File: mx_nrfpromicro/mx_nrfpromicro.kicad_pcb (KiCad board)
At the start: 2 copper layers, 22 parts, among them SW1 SW_Push_45deg, SW10 SW_Push_45deg, SW11 SW_Push_45deg, SW12 SW_Push_45deg, SW13 SW_Push_45deg, SW14 SW_Push_45deg, SW15 SW_Push_45deg, SW16 SW_Push_45deg, SW17 SW_Push_45deg, SW2 SW_Push_45deg, SW3 SW_Push_45deg, SW4 SW_Push_45deg, SW5 SW_Push_45deg, SW6 SW_Push_45deg, SW7 SW_Push_45deg, SW8 SW_Push_45deg, SW9 SW_Push_45deg, U1 Nice_Nano_V2

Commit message: updated
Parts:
- SW18: value ~ -> SW_SPDT
- SW19: value ~ -> SW_PUSH
- moved SW11 292.3 mm to (38.1, 90.8)
- moved SW13 278.2 mm to (76.2, 75.8)
- moved SW7 275.9 mm to (57.1, 59.8)
- moved SW1 275.3 mm to (38.1, 52.7)
- moved SW6 274.6 mm to (38.1, 71.8)
- moved SW12 273.7 mm to (57.1, 78.8)
- moved SW14 258.2 mm to (95.2, 83.8)
- moved SW8 254.9 mm to (76.2, 56.8)
- moved SW2 254.5 mm to (57.1, 40.7)
- moved SW16 249.9 mm to (102.1, 105.9), turned to -12 degrees
- moved SW18 249.2 mm to (136.5, 88.7), turned to -90 degrees
- moved TP2 245.5 mm to (125.6, 39.7)
- moved SW19 244.8 mm to (140.6, 76.7), turned to 90 degrees
- moved SW15 237.2 mm to (114.3, 86.0)
- moved U1 236.2 mm to (133.1, 56.0)
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
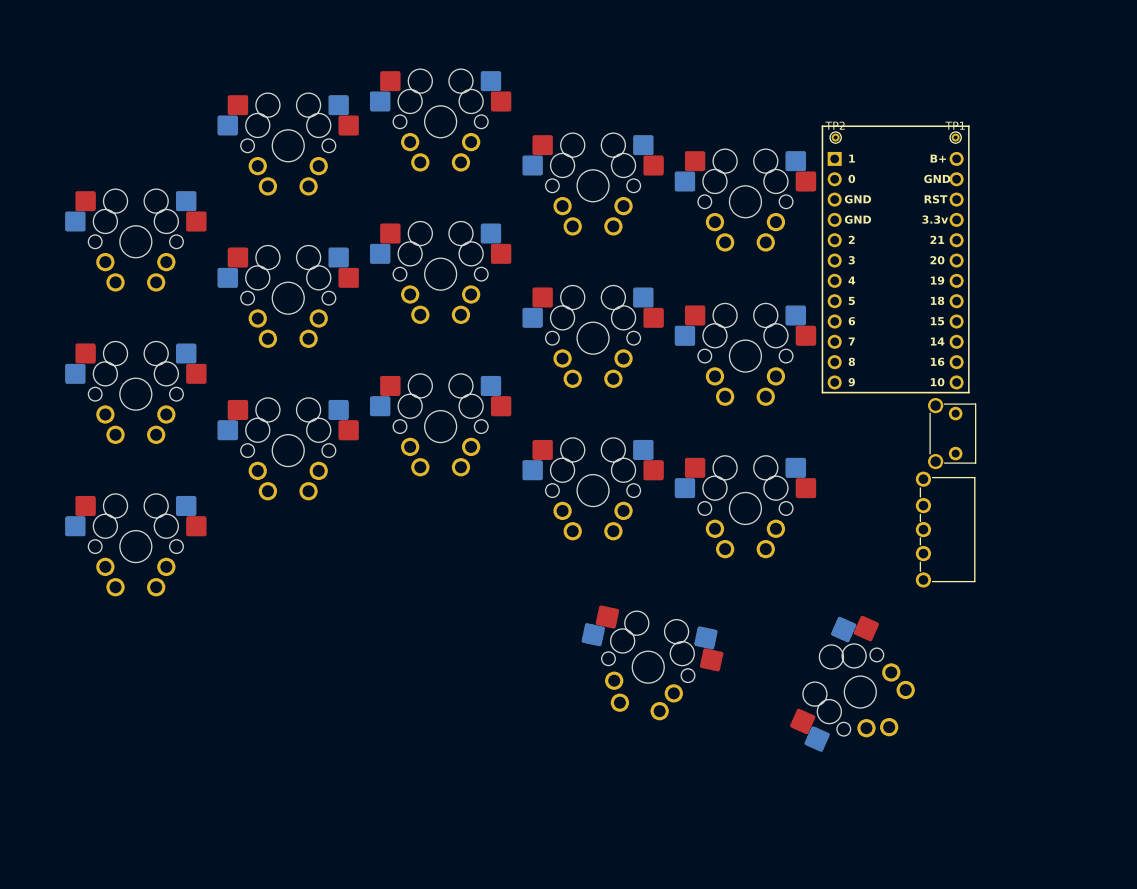
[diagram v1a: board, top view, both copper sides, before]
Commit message: updated
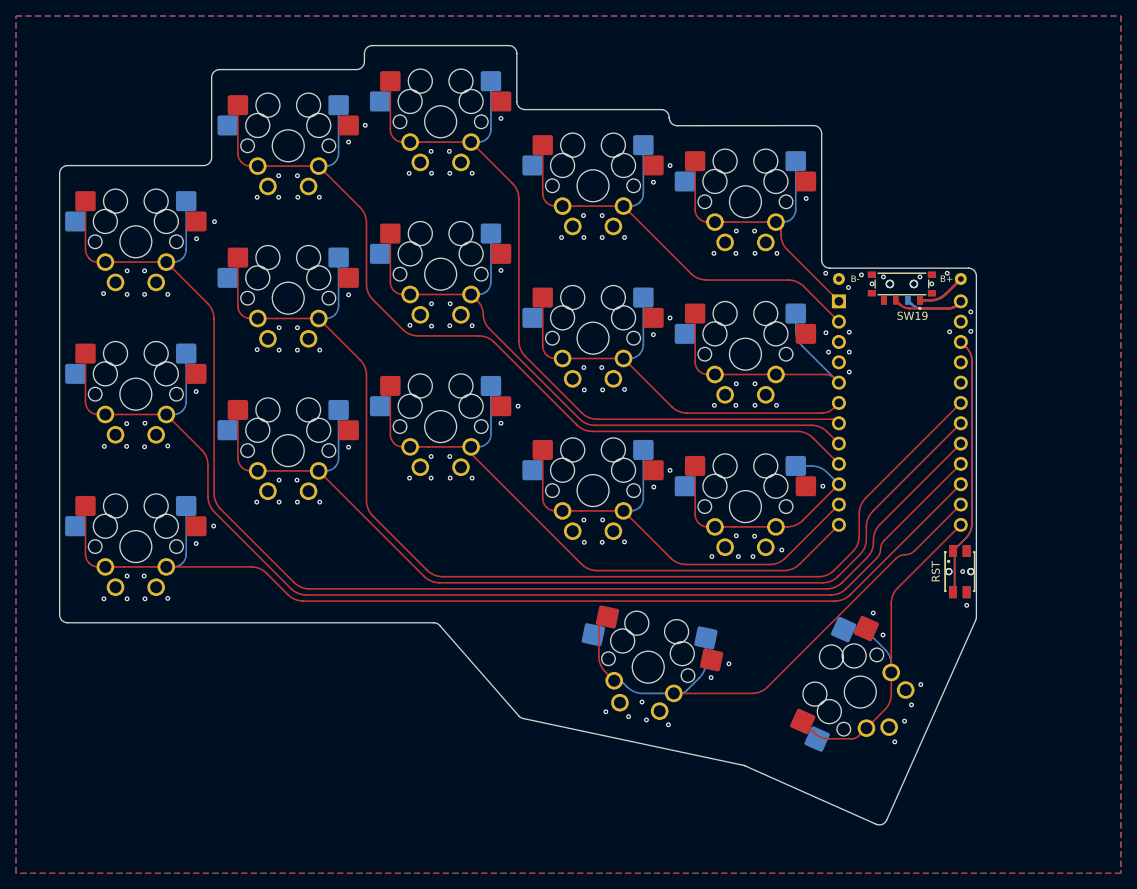
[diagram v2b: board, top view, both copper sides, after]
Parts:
- added RST: 436331045822, BLE_KBD:4363X10458XX, F.Cu at (141.1, 93.9)
- added RST: 436331045822, BLE_KBD:4363X10458XX, B.Cu at (141.1, 93.9)
- B+: renamed from TP1; footprint TestPoint:TestPoint_THTPad_D1.0mm_Drill0.5mm -> TestPoint:TestPoint_THTPad_D1.5mm_Drill0.7mm
- B-: renamed from TP2; footprint TestPoint:TestPoint_THTPad_D1.0mm_Drill0.5mm -> TestPoint:TestPoint_THTPad_D1.5mm_Drill0.7mm
- SW1, SW10, SW11, SW12, SW13, SW14, SW15, SW2, SW3, SW4, SW5, SW6, SW7, SW8, SW9: footprint BLE_KBD:MX_Optional_Reversible_1u -> BLE_KBD:MX_Reversible_Optional_1u
- SW16, SW17: footprint BLE_KBD:MX_Optional_Reversible_1.5u -> BLE_KBD:MX_Reversible_Optional_1.5u
- SW18: value SW_SPDT -> MLL1200S; footprint BLE_KBD:SS12F23G5 -> BLE_KBD:SW_MLL1200S; moved to B.Cu
- SW19: value SW_PUSH -> MLL1200S; footprint BLE_KBD:SW_SIDE_MOUNT -> BLE_KBD:SW_MLL1200S
- moved SW18 30.8 mm to (133.9, 58.0), turned to 0 degrees
- moved SW19 19.9 mm to (133.9, 58.0), turned to 180 degrees
- moved U1 17.8 mm to (133.6, 73.8)
- moved B+ 17.7 mm to (141.2, 57.4)
- moved B- 17.7 mm to (126.0, 57.4)
- moved SW10 0.24 mm to (114.3, 66.8)
- moved SW15 0.24 mm to (114.3, 85.8)
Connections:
- B+ pad 1: Net-(SW18-Pad2) -> Net-(SW18-Pad3)
- SW18 pad 1: Net-(U1-B+) -> unconnected-(SW18-Pad1)
- SW18 pad 2: Net-(SW18-Pad2) -> B+
- SW18 pad 3: unconnected-(SW18-Pad3) -> Net-(SW18-Pad3)
- SW19 pad 1: RST -> Net-(SW18-Pad3)
- SW19 pad 2: GND -> B+
- SW19 pad 3: GND -> unconnected-(SW19-Pad3)
- U1 pad 1: SW1 -> SW5
- U1 pad 10: SW8 -> SW15
- U1 pad 11: SW9 -> SW14
- U1 pad 12: SW10 -> SW13
- U1 pad 13: SW11 -> SW17
- U1 pad 14: SW12 -> SW16
- U1 pad 15: SW13 -> SW11
- U1 pad 16: SW14 -> SW6
- U1 pad 17: SW15 -> SW1
- U1 pad 18: SW16 -> SW12
- U1 pad 19: SW17 -> SW7
- U1 pad 2: SW2 -> SW4
- U1 pad 24: Net-(U1-B+) -> B+
- U1 pad 5: SW3 -> SW10
- U1 pad 6: SW4 -> SW9
- U1 pad 7: SW5 -> SW3
- U1 pad 8: SW6 -> SW8
- U1 pad 9: SW7 -> SW2
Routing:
- net SW1: track 0.00 -> 165.0 mm
- net SW6: track 0.00 -> 145.6 mm
- net SW7: track 0.00 -> 141.8 mm
- net SW11: track 0.00 -> 133.2 mm
- net SW12: track 0.00 -> 122.5 mm
- net SW2: track 0.00 -> 111.9 mm
- net SW3: track 0.00 -> 98.3 mm
- net SW13: track 0.00 -> 81.2 mm
- net SW8: track 0.00 -> 80.8 mm
- net SW16: track 0.00 -> 71.4 mm
- net RST: track 0.00 -> 65.3 mm
- net SW14: track 0.00 -> 59.5 mm
- net SW4: track 0.00 -> 59.1 mm
- net SW9: track 0.00 -> 56.4 mm
- net SW17: track 0.00 -> 48.4 mm
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- added copper zone on B.Cu, net GND
- added copper zone on F.Cu, net GND
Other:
- board outline added: 114.6 x 97.4 mm
